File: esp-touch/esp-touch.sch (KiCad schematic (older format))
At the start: 60 parts, among them P1 CONN_01X02, P2 CONN_01X05, P3 DISPLAY, P4 CONN_01X03, P5 CONN_01X02, P6 CONN_01X02, P7 CONN_01X04, Q1 Q_NMOS_GSD, SW1 SW_PUSH_SMALL, SW2 SW_PUSH_SMALL, U1 ESP-12E, U2 AP2114H-3.3, U3 SI7021, U4 FT231XS, U5 MPR121Q

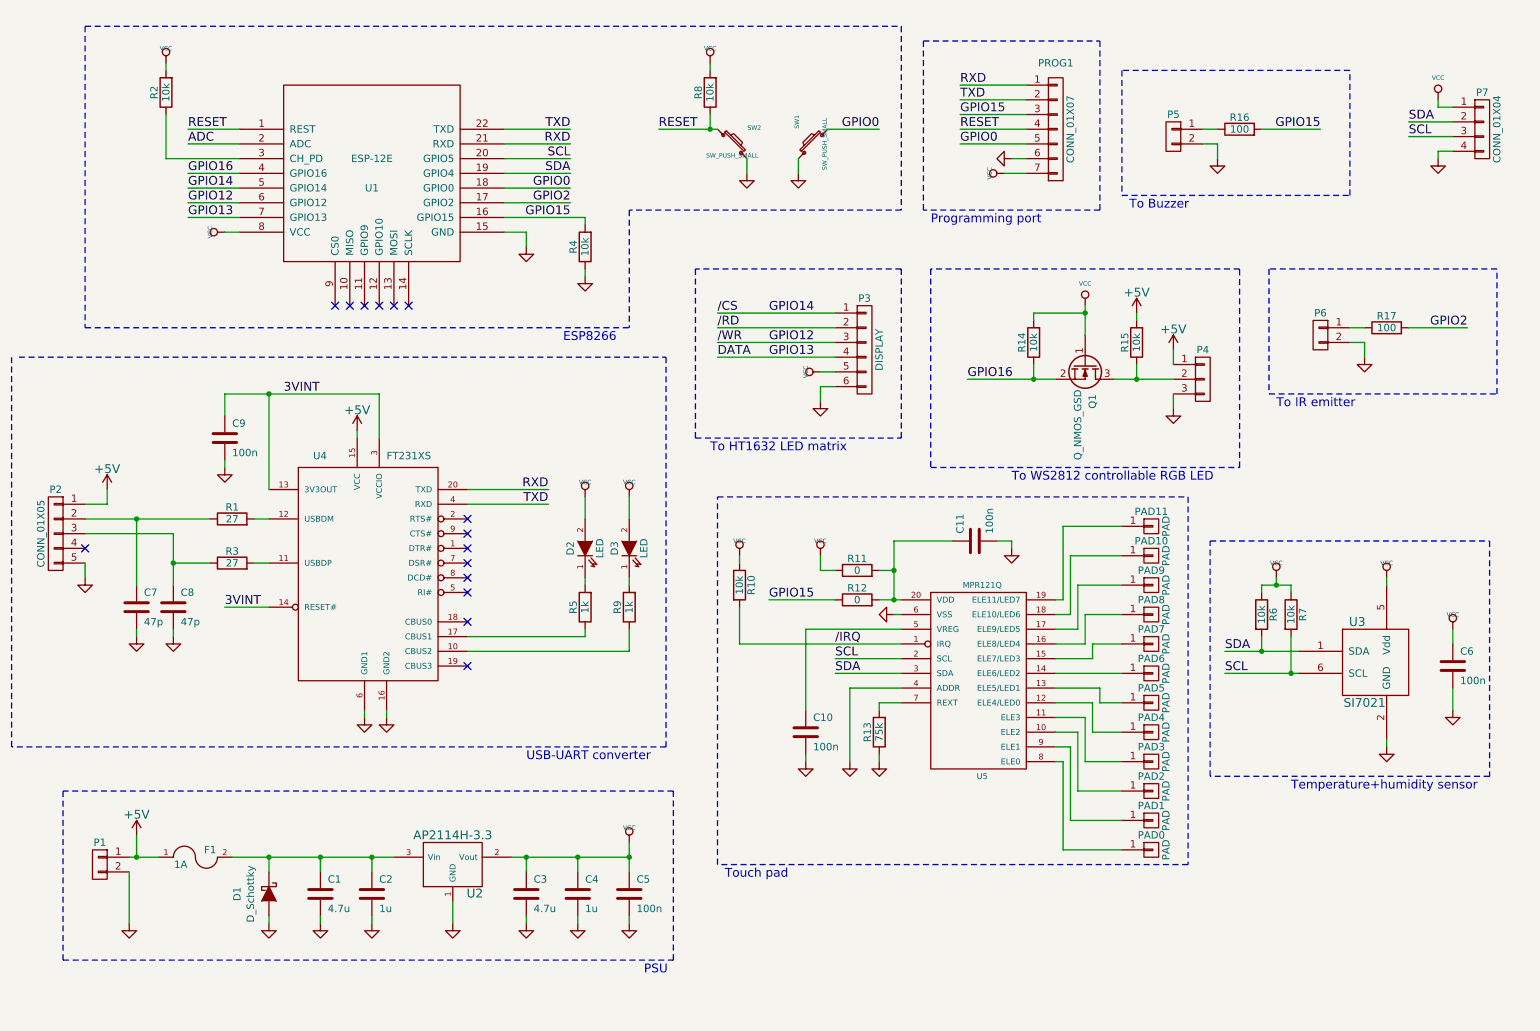
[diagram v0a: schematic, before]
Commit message: Multiple mistakes fixed
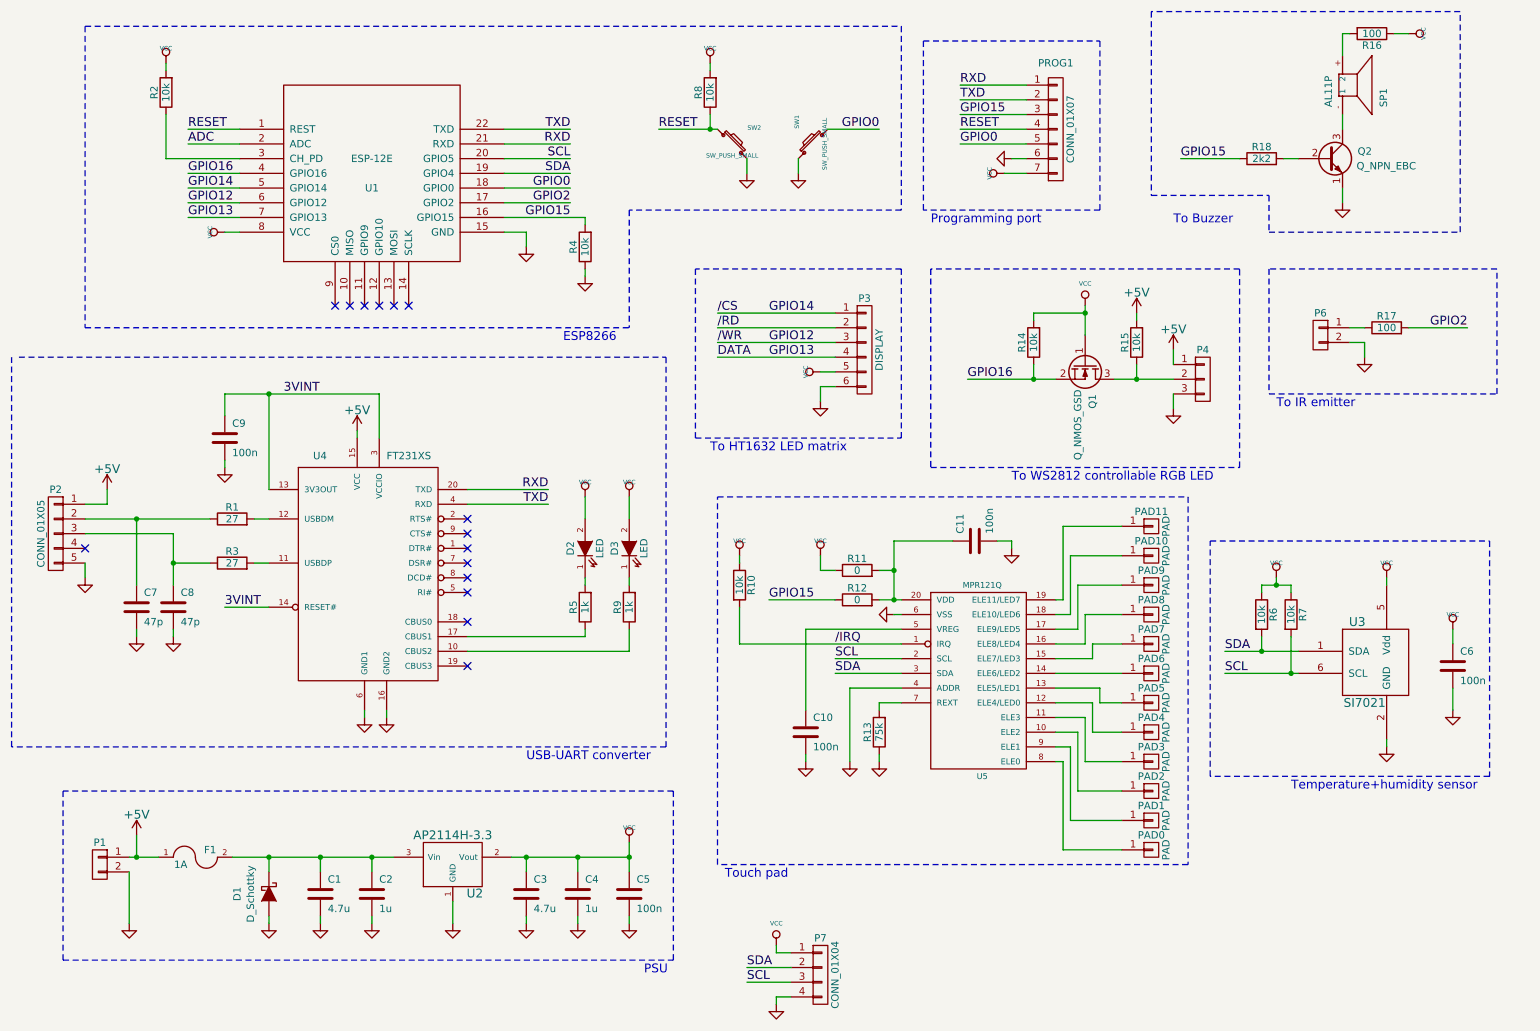
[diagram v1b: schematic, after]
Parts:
- removed P5: CONN_01X02, Pin_Headers:Pin_Header_Straight_1x02, symbol CONN_01X02
- added Q2: Q_NPN_EBC, mysmd:SOT23EBC, symbol Q_NPN_EBC
- added R18: 2k2, mysmd:SM0603S, symbol R
- added SP1: AL11P, mymods:Buzzer_7.6_12.0, symbol AL11P
- P2: footprint mysmd:microUSB_female -> mysmd:MICRO_USB_SOCKET
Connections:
- net GND: now also Q2.1 (E)
- net GPIO15: now also R18.1; no longer R16.2
- net VCC: now also R16.1
- new net: R16.2, SP1.+ (2)
- new net: Q2.2 (B), R18.2
- new net: Q2.3 (C), SP1.- (1)
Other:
- moved on the sheet: P7, R16
